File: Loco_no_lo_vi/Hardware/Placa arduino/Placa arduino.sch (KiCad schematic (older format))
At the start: 27 parts

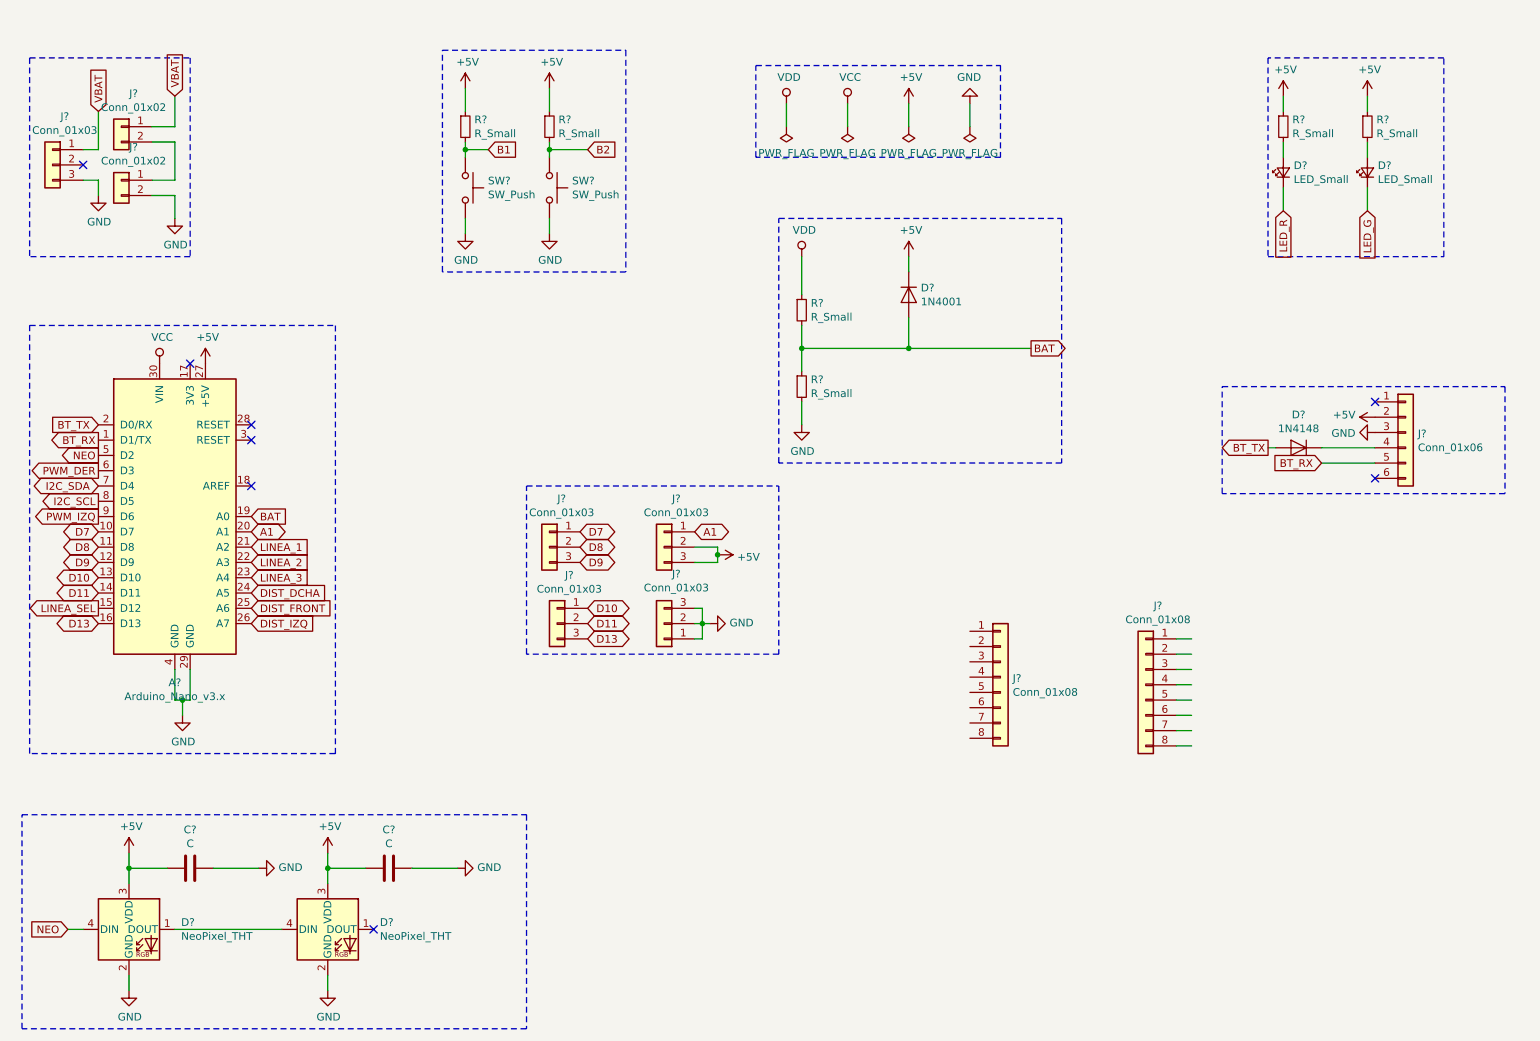
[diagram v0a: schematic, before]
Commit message: Más esquema
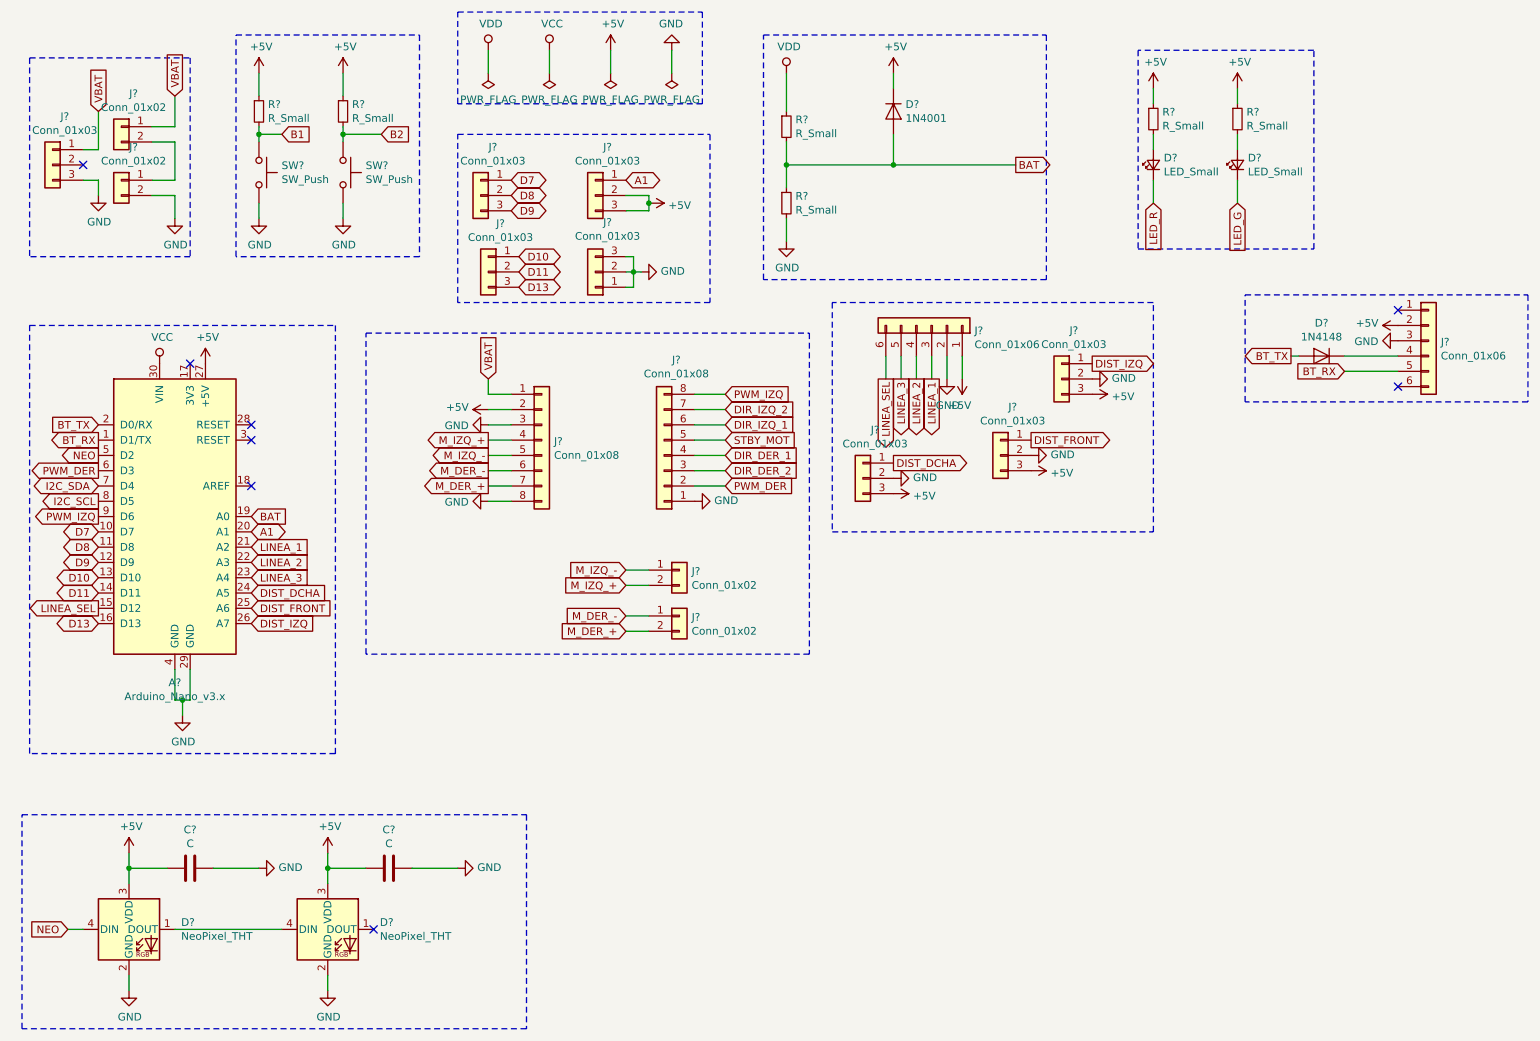
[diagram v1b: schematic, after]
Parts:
- removed J? (x2): Conn_01x08, symbol Connector_Generic:Conn_01x08
- added J? (x2): Conn_01x08, symbol Connector_Generic:Conn_01x08
- added J? (x2): Conn_01x02, symbol Connector_Generic:Conn_01x02
- added J?: Conn_01x06, symbol Connector_Generic:Conn_01x06
- added J? (x3): Conn_01x03, symbol Connector_Generic:Conn_01x03
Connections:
- net labels added: DIR_DER_1, DIR_DER_2, DIR_IZQ_1, DIR_IZQ_2, M_DER_+, M_DER_-, M_IZQ_+, M_IZQ_-, STBY_MOT
- wire segments 77 -> 95
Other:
- moved on the sheet: D?, J?, R?, SW?
